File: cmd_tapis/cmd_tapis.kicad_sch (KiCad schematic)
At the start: 12 parts, among them X1 Trou, X2 Trou, X3 Trou, X4 Trou

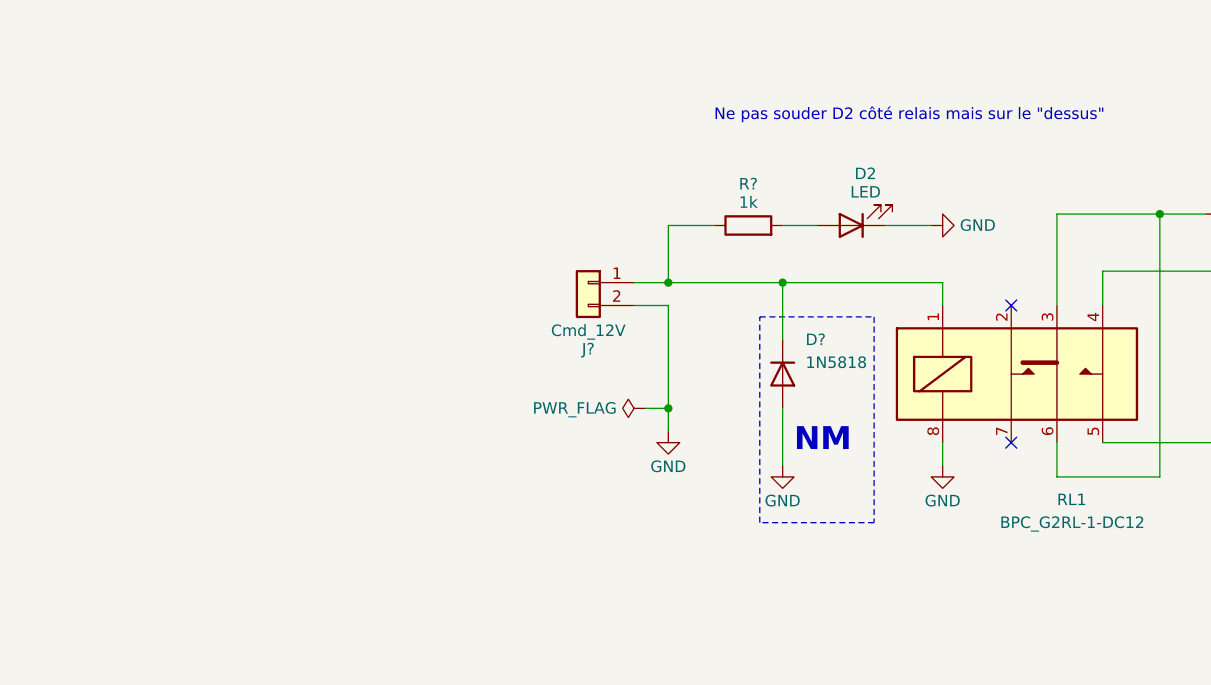
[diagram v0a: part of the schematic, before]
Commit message: Améliorations:
- Isolation renforcée en coupant le PCB
- Ajout de passage pour colliers de serrage des cables
- Ajout diode en direct
- Ajout découplages
- Alignement grille 1mm
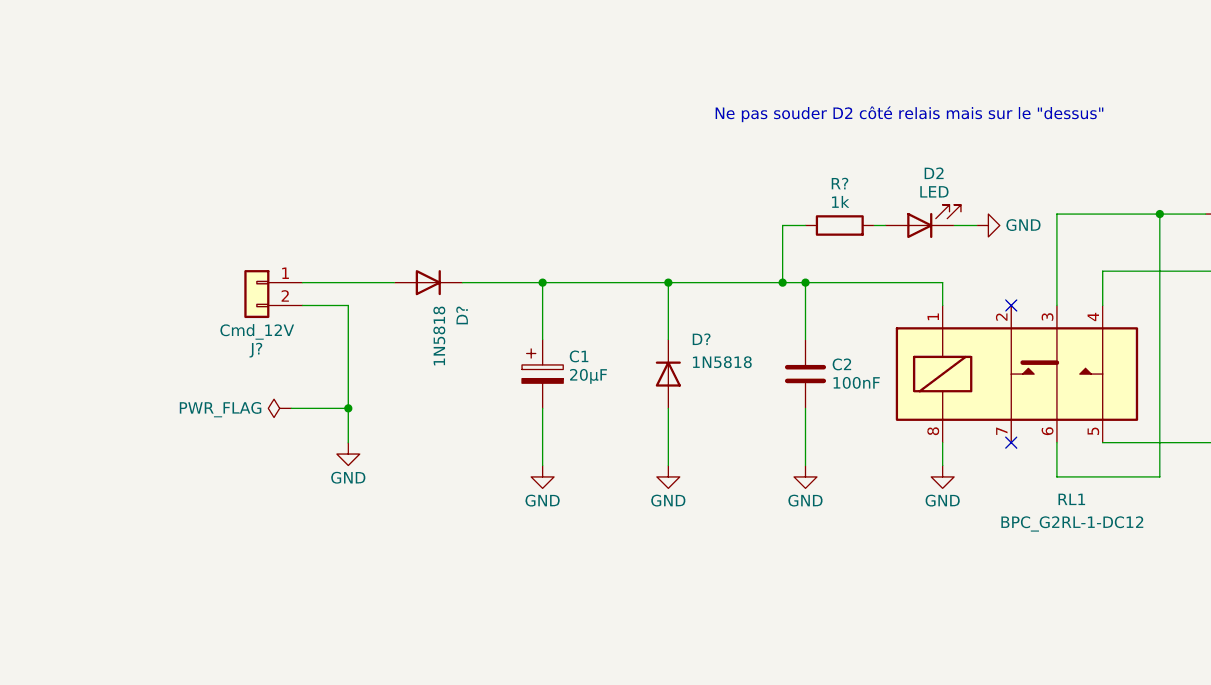
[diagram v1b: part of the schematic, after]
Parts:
- added C1: 20µF, Capacitor_THT:CP_Radial_D5.0mm_P2.50mm, symbol Device:C_Polarized
- added C2: 100nF, Capacitor_THT:C_Disc_D3.8mm_W2.6mm_P2.50mm, symbol Device:C
- added D?: 1N5818, Diode_THT:D_A-405_P10.16mm_Horizontal, symbol Device:D
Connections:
- net GND: now also C1.2, C2.2
- net at D?.1 (K), R?.1, RL1.1: now also C1.1, C2.1, D?.1 (K); no longer J?.1 (Pin_1)
- new net: D?.2 (A), J?.1 (Pin_1)
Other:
- note removed: "NM"
- moved on the sheet: D2, D?, J?, R?
